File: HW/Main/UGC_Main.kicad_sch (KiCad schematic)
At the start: 147 parts, among them J1 Rumble, J1 USB4105-GF-A-060, J10 Conn_01x01_Pin, J11 Conn_01x01_Pin, J12 Conn_01x01_Pin, J2 LT, J3 RT, J5 Conn_01x01_Pin, J6 Conn_01x01_Pin, J7 Conn_01x01_Pin, J7 Conn_01x05_Pin, J8 Conn_01x01_Pin, J9 Conn_01x01_Pin, J9 Conn_01x05_Pin, Q1 MMBT3904, Q2 MMBT3904, Q3 BSS138DW, Q4 BSS138DW, Q5 Q_NMOS_GSD, Q6 Q_PMOS_GDS, Q7 Q_NMOS_GSD, SW1 SW_Push, SW10 SW_Push, SW11 SW_Push, SW12 SW_Push, SW13 SW_Push, SW14 TS09-63-25-R-260-SMT, SW2 SW_Push, SW3 SW_Push, SW4 SW_Push, SW5 SW_Push, SW6 GL18_SW, SW7 SW_Push, SW8 SW_Push, SW9 TS09-63-25-R-260-SMT, T1 36-8730, T2 36-8730, T3 36-8730, T4 36-8730, U1 ESP32-PICO-MINI-02, U10 ST_LSM6, U11 BQ25180, U12 CH340K, U13 PI3USB4000A, U14 GH39F (Hall SOT23), U15 GH39F (Hall SOT23), U16 GH39F (Hall SOT23), U17 GH39F (Hall SOT23), U2 GD25Q80EEIGR, U2 GH39F (Hall SOT23), U3 GH39F (Hall SOT23), U4 GH39F (Hall SOT23), U5 GH39F (Hall SOT23), U6 MCP3002, U7 MCP3002, U8 RP2040, Y1 Crystal_GND3

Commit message: Checkpoint 2
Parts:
- removed C23, C24, C25, C26, C4: .047u, Capacitor_SMD:C_0603_1608Metric_Pad1.08x0.95mm_HandSolder, symbol Device:C
- removed J7: Conn_01x05_Pin, hhl:molex_5034800540, symbol Connector:Conn_01x05_Pin
- removed J9: Conn_01x05_Pin, Connector_PinHeader_2.00mm:PinHeader_1x05_P2.00mm_Vertical, symbol Connector:Conn_01x05_Pin
- removed L2, L4, L6, L8: SK6805-EC-15, hhl:SK6805-EC-15, symbol progcc_v3:SK6805-EC-15
- removed R3, R39: 1k, Resistor_SMD:R_0201_0603Metric, symbol Device:R
- removed T1: 36-8730, hhl:KS_8730, symbol Connector:TestPoint
- removed T2, T3, T4: 36-8730, progcc_v3:KS_8730, symbol Connector:TestPoint
- removed TP1, TP2, TP3: TestPoint, TestPoint:TestPoint_Pad_D1.5mm, symbol Connector:TestPoint
- removed U14, U15, U16, U17, U4, U5: GH39F (Hall SOT23), progcc_v3:GH39F, symbol progcc_v3:GH39F (Hall SOT23)
- added C1: 47uF 6.3v, Capacitor_Tantalum_SMD:CP_EIA-3216-18_Kemet-A, symbol Device:C_Polarized
- added C2: 2.2uF, Capacitor_SMD:C_0603_1608Metric, symbol Device:C
- added D10, D9: CUS08F30, Diode_SMD:D_SOD-323_HandSoldering, symbol progcc_v3:CUS08F30
- added F1: Fuse, Fuse:Fuse_1206_3216Metric_Pad1.42x1.75mm_HandSolder, symbol Device:Fuse
- added J13: 503480-0640, hhl:5034800640, symbol hhl:503480-0640
- added J4: Conn_01x06_Pin, Connector_PinHeader_2.00mm:PinHeader_1x06_P2.00mm_Vertical, symbol Connector:Conn_01x06_Pin
- added R14: 10k, Resistor_SMD:R_0201_0603Metric, symbol Device:R_Small
- added TP5: TestPoint, TestPoint:TestPoint_Pad_D1.5mm, symbol Connector:TestPoint
- added U3: XC6222, hhl:SOT-89-5, symbol hhl:XC6222B331PR-G
- added U5: ST_LSM6, hhl:LGA14, symbol progcc_v3:ST_LSM6
- C3: value .047u -> 2.2uF; footprint Capacitor_SMD:C_0603_1608Metric_Pad1.08x0.95mm_HandSolder -> Capacitor_SMD:C_0603_1608Metric; LCSC C15849 -> (none)
- R36, R37, R38, R4: value 1k -> 75k; footprint Resistor_SMD:R_0201_0603Metric -> Resistor_SMD:R_0603_1608Metric
- U2, U3: footprint progcc_v3:GH39F -> hhl:GH39F
- renumbered L3 to L2, L5 to L3, L7 to L4
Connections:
- net LS_BUTTON is gone; now on net Pulldown_D: SW6.S1 (1), SW6.S2 (2)
- net SR_Pull is gone; now on net DD_Pull: D4.6 (K)
- net UART0_TX is gone; now on net VBUS_SYS: JP1.2 (B)
- net VBUS_PRE is gone; now on net +5V_PRE: D1.2 (A)
- net +3V3: now also R36.2, R38.2, RV1.1 (GND), RV2.1 (GND), C1.1, C2.1, D10.2 (A), D9.1 (K), J13.6, J4.6 (Pin_6), TP5.1, U3.5 (Vout), U5.5 (VDDIO), U5.8 (VDD)
- net +5V: now also C16.1, D1.1 (K), JP1.1 (A), U11.A2 (IN); no longer J1.A4_B9 (VBUS), J1.B4_A9 (VBUS)
- net A_Pull: now also D1.6 (K), SW1.2; no longer D3.4 (K)
- net BAT_LVL: now also U8.40 (GPIO28_ADC2); no longer JP1.1 (A), U8.38 (GPIO26_ADC0)
- net BTN_PWR: now also U8.7 (GPIO5); no longer U8.16 (GPIO13)
- net B_Pull: now also D2.5 (K), SW2.2; no longer D5.6 (K)
- net D+: now also J7.1 (Pin_1)
- net D-: now also J9.1 (Pin_1)
- net DD_Pull: now also SW11.2; no longer D3.5 (K)
- net DL_Pull: now also D2.4 (K), SW12.2; no longer D5.5 (K)
- net DR_Pull: now also D5.5 (K), SW13.2; no longer D4.4 (K)
- net DU_Pull: now also D1.5 (K), SW10.2; no longer D2.6 (K)
- net ESP_EN: now also U8.38 (GPIO26_ADC0); no longer U8.18 (GPIO15)
- net GND: now also J5.1 (Pin_1), R37.1, R4.1, RV1.3 (V+), RV2.3 (V+), SW9.2, C1.2, C2.2, J13.1, J13.MP1, J13.MP2, J4.1 (Pin_1), U3.2 (GND), U5.2 (SDx), U5.3 (SCx), U5.6 (GNDIO), U5.7 (GND)
- net I2C_SCL: now also U8.35 (GPIO23); no longer U8.3 (GPIO1)
- net I2C_SDA: now also U8.34 (GPIO22); no longer U8.2 (GPIO0)
- net IMU0_CS: now also U8.2 (GPIO0); no longer U8.28 (GPIO17)
- net IMU1_CS: now also U8.4 (GPIO2), U5.12 (CS); no longer U8.32 (GPIO21)
- net LADC_CS: now also U8.3 (GPIO1); no longer U8.27 (GPIO16)
- net LX: no longer R36.2
- net LY: no longer R37.2
- net L_Pull: now also D1.4 (K), SW7.2; no longer D5.4 (K)
- net N_CLOCK: now also J6.1 (Pin_1)
- net N_CLOCK_3.3: now also U8.31 (GPIO20); no longer U8.5 (GPIO3)
- net N_DATA: now also J8.1 (Pin_1)
- net N_DATA_3.3: now also U8.30 (GPIO19); no longer U8.4 (GPIO2)
- net N_LATCH: now also J10.1 (Pin_1)
- net N_LATCH_3.3: now also U8.29 (GPIO18); no longer U8.6 (GPIO4)
- net Plus_Pull: now also D3.5 (K), SW5.2; no longer D1.5 (K)
- net RADC_CS: now also U8.12 (GPIO9); no longer U8.34 (GPIO22)
- net RGB_OUT: now also U8.32 (GPIO21); no longer U8.35 (GPIO23)
- net RUMBLE: now also U8.5 (GPIO3); no longer U8.36 (GPIO24)
- net RUMBLE-: now also J1.2 (Pin_2)
- net RX: now also J13.5, J4.5 (Pin_5); no longer C3.2, R38.2
- net RY: now also J13.4, J4.4 (Pin_4); no longer R4.2
- net R_BRAKE: now also U8.6 (GPIO4); no longer U8.37 (GPIO25)
- net R_Pull: now also D4.5 (K), SW8.2; no longer D3.6 (K)
- net SHARED_PU: now also D10.1 (K)
- net SL_Pull: now also D2.6 (K), SW6.S3 (3), SW6.S4 (4); no longer D2.4 (K)
- net SPI_CK: now also U8.8 (GPIO6), U5.13 (SCL); no longer U8.29 (GPIO18)
- net SPI_RX: now also U8.11 (GPIO8), U5.1 (SDO); no longer U8.31 (GPIO20)
- net SPI_TX: now also U8.9 (GPIO7), U5.14 (SDA); no longer U8.30 (GPIO19)
- net Scan_A: now also D1.1 (A), D1.2 (A), D1.3 (A), D2.1 (A), U8.16 (GPIO13); no longer U8.15 (GPIO12)
- net Scan_B: now also D2.2 (A), D2.3 (A), D3.1 (A), D3.2 (A), U8.15 (GPIO12); no longer U8.12 (GPIO9)
- net Scan_C: now also D3.3 (A), D4.1 (A), D4.2 (A), D4.3 (A), U8.14 (GPIO11); no longer U8.8 (GPIO6)
- net Scan_D: now also D5.1 (A), D5.2 (A), D5.3 (A), U8.13 (GPIO10); no longer U8.11 (GPIO8)
- net USB_EN: now also U8.36 (GPIO24); no longer U8.41 (GPIO29_ADC3)
- net USB_SEL: now also U8.37 (GPIO25); no longer U8.17 (GPIO14)
- net VBUS_SYS: now also C3.2, J1.1 (Pin_1), R14.2, U3.4 (Vin)
- net X_Pull: now also D3.4 (K), SW3.2; no longer D1.6 (K)
- net Y_Pull: now also D5.6 (K), SW4.2; no longer D2.5 (K)
- net ZL_ANALOG: now also R36.1, R4.2, RV1.2 (Signal), U8.41 (GPIO29_ADC3); no longer U8.39 (GPIO27_ADC1)
- net ZL_Pull: now also D3.6 (K), J2.1 (Pin_1); no longer D1.4 (K)
- net ZR_ANALOG: now also R37.2, R38.1, RV2.2 (Signal), U8.39 (GPIO27_ADC1); no longer U8.40 (GPIO28_ADC2)
- net ZR_Pull: now also D5.4 (K), J3.1 (Pin_1); no longer D4.5 (K)
- net Pulldown_C: now reaches J3.2 (Pin_2)
- net Pulldown_C: now also J2.2 (Pin_2), SW7.1, SW8.1, U8.27 (GPIO16)
- net Pulldown_A: now reaches SW1.1
- net Pulldown_A: now also SW2.1, SW3.1, SW4.1, U8.17 (GPIO14)
- net Pulldown_B: now reaches SW12.1
- net Pulldown_B: now also SW10.1, SW11.1, SW13.1, U8.18 (GPIO15)
- net +3V3_PRE: now reaches J12.1 (Pin_1)
- net +3V3_PRE: now also F1.2
- net +5V_PRE: now reaches J11.1 (Pin_1)
- net +5V_PRE: now also J1.A4_B9 (VBUS), J1.B4_A9 (VBUS)
- net Pulldown_D: now reaches SW5.1
- net Pulldown_D: now also U8.28 (GPIO17), J13.3, J4.3 (Pin_3)
- removed net Push_A: D1.1 (A), D1.2 (A), D1.3 (A), D2.1 (A), U8.7 (GPIO5)
- removed net Push_B: D2.2 (A), D2.3 (A), D3.1 (A), D3.2 (A), U8.9 (GPIO7)
- removed net Push_C: D3.3 (A), D4.1 (A), D4.2 (A), D4.3 (A), U8.13 (GPIO10)
- removed net Push_D: D5.1 (A), D5.2 (A), D5.3 (A), U8.14 (GPIO11)
- new net: R14.1, U3.1 (CE)
- new net: D9.2 (A), F1.1
- new net RS_B_IN: D4.4 (K), J13.2, J4.2 (Pin_2)
- no-connect marks 4 -> 8
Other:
- note added: "IMU 1"
- note added: "Input Matrix: One of the pulldowns is pulled to ground or set LOW. The others are set HIGH. When a button is pressed, the corresponding SCAN pin is pulled low, allowing for an indication of which button has been pressed according to which pulldown pin is active."
- note added: "LS"
- note added: "Power Bus"
- note removed: "Rumble Connection"
- moved on the sheet: C1, C10, C2, D1A, D1B, D1C, D2A, D2B, D2C, D3A, D3B, D3C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

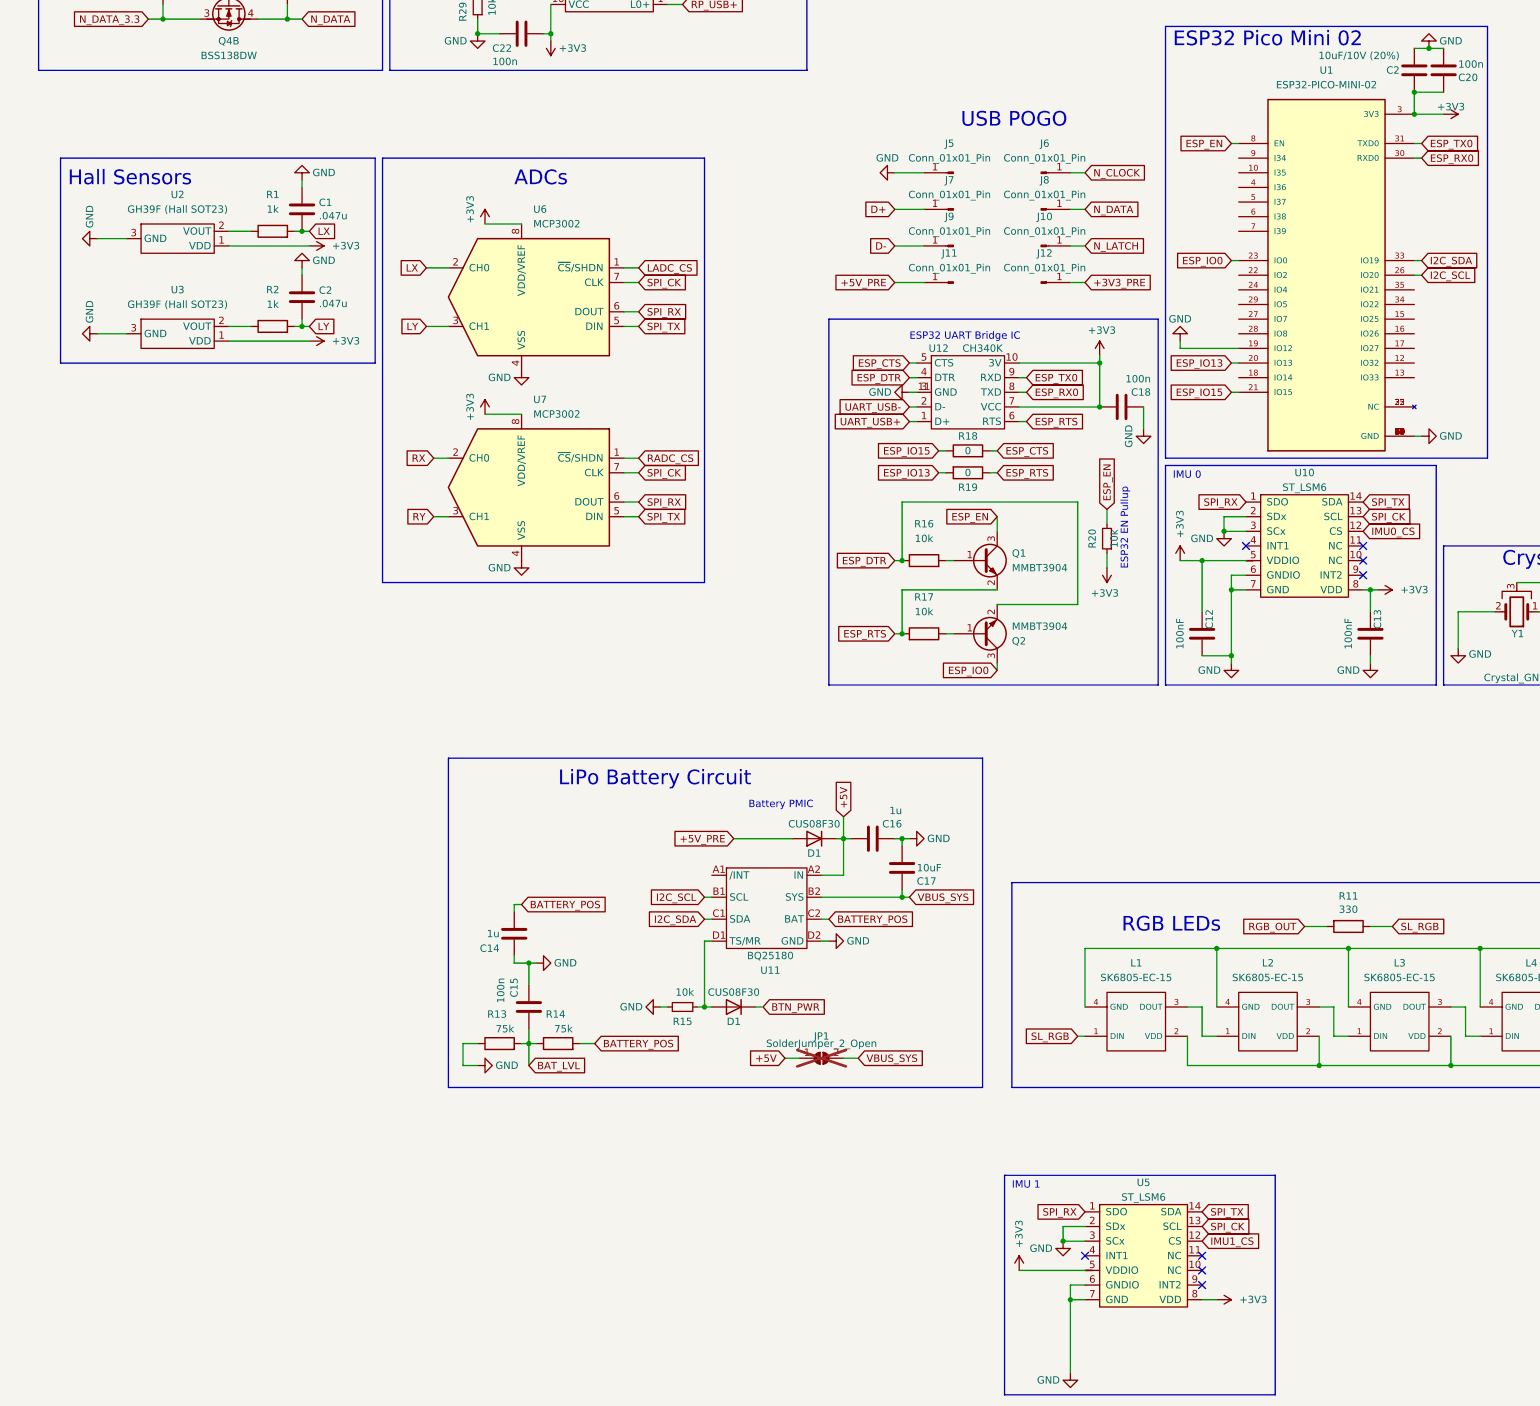
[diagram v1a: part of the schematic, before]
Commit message: Updates
- Stick PCB
- USB C pcb
- trigger PCB
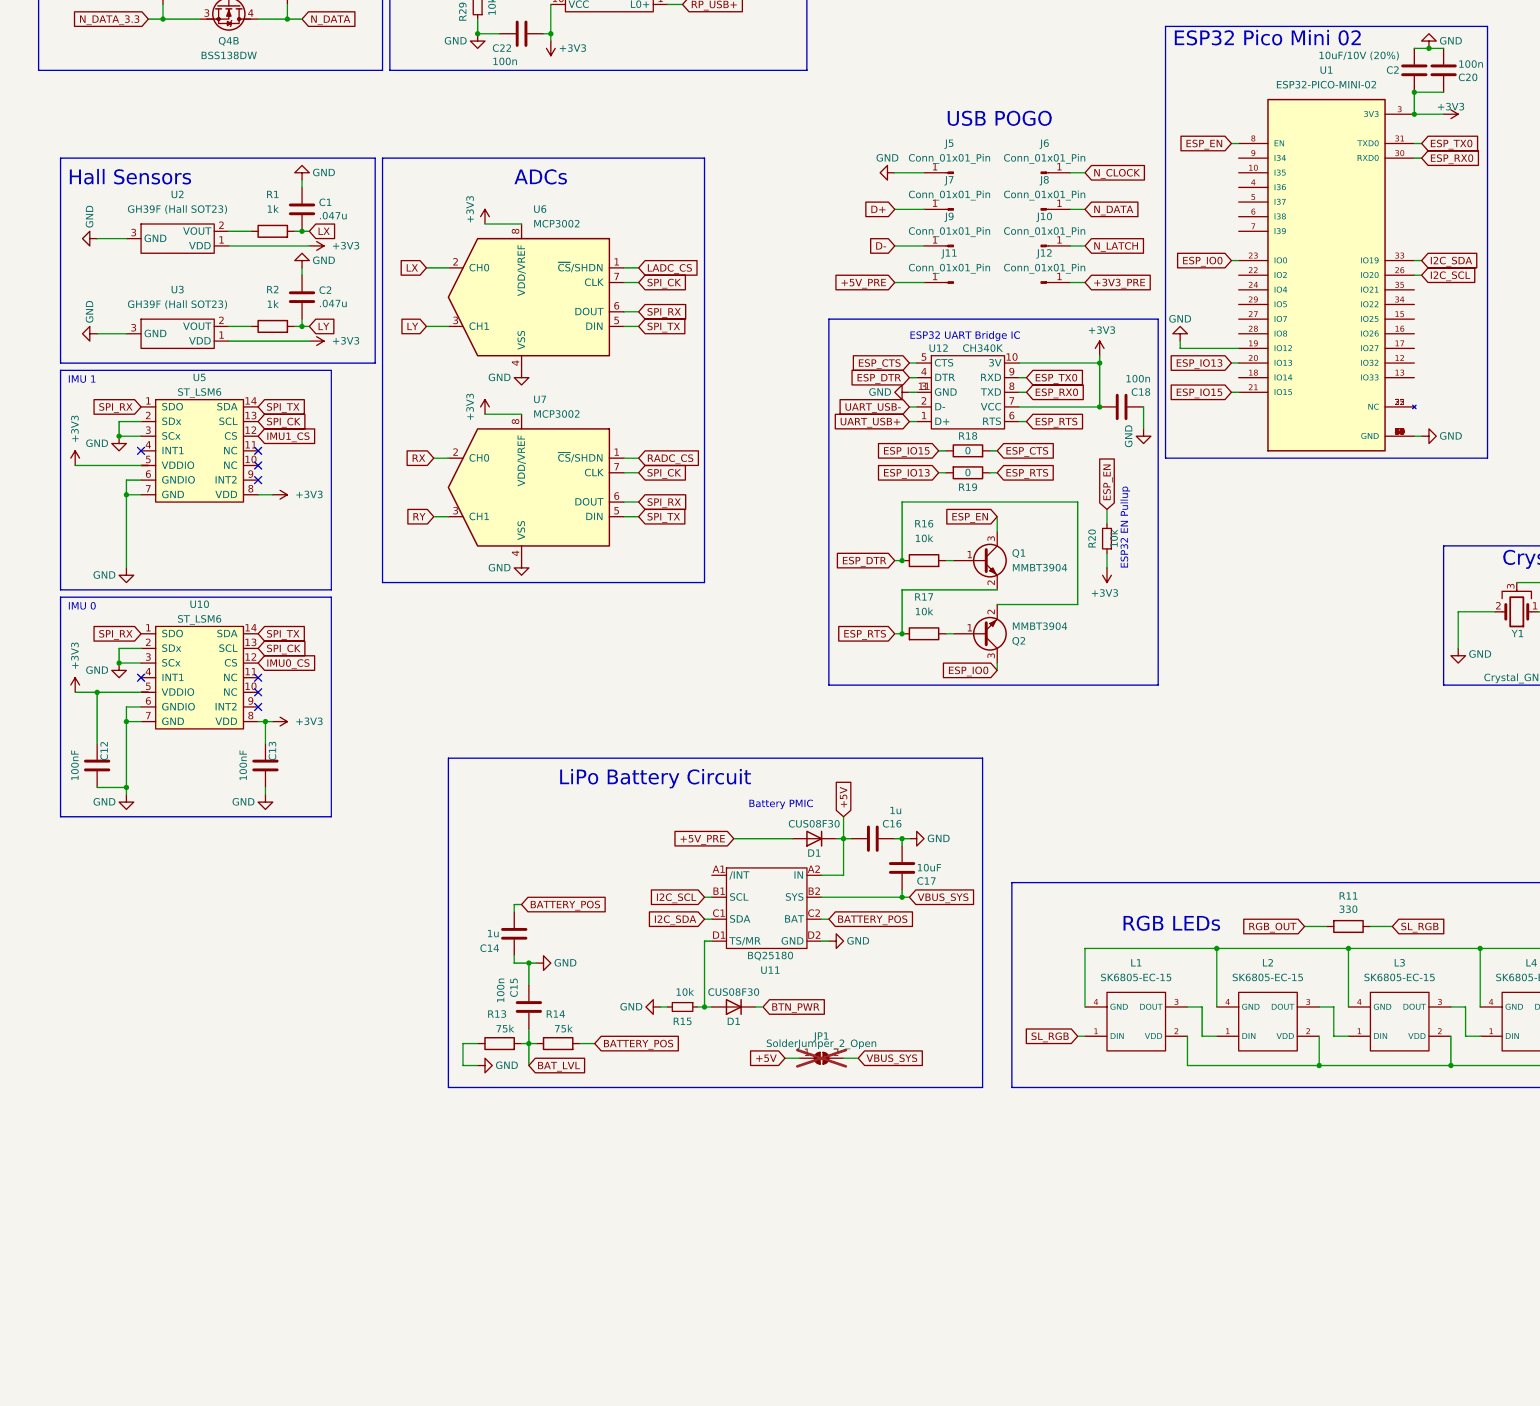
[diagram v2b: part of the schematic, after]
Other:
- moved on the sheet: C12, C13, U10, U5

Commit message: Production files
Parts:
- J1, J2, J3, SW1, SW10, SW11, SW12, SW13, SW2, SW3, SW4, SW5: now not fitted; now left out of the parts list
- J10, J11, J12, J5, J6, J7, J8, J9: MPN (none) -> YZ72015053P-01
- J13: MPN (none) -> 503480-0640; Manufacturer_Part_Number 503480-0640 -> (none)
- SW7, SW8: MPN (none) -> TC-00100V H5.0 100gf
- U1: MPN (none) -> ESP32-PICO-MINI-02
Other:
- note added: "Analog Triggers"
- note added: "Internal USB"
- moved on the sheet: B1, C1, C12, C13, C14, C15, C16, C17, C18, C2, C20, C21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
